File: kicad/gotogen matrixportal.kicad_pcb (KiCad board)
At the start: 2 copper layers, 139.7 x 63.5 mm, 27 parts, among them J1 HUB75 Out, J2 HUB75 In, J3 OLED_128_64, J4 Buttons EXT, J5 OpenMV, J6 Extra Connections, J7 Capacitive Touch, SW1 Back, SW2 Menu, SW3 Up, SW4 Down, SW5 Extra1, SW6 Extra2, U1 MatrixPortal_M4, U2 PCF8523_Breakout, U3 PCF8574, U4 MPR121_Breakout, U5 MAX9814_Breakout

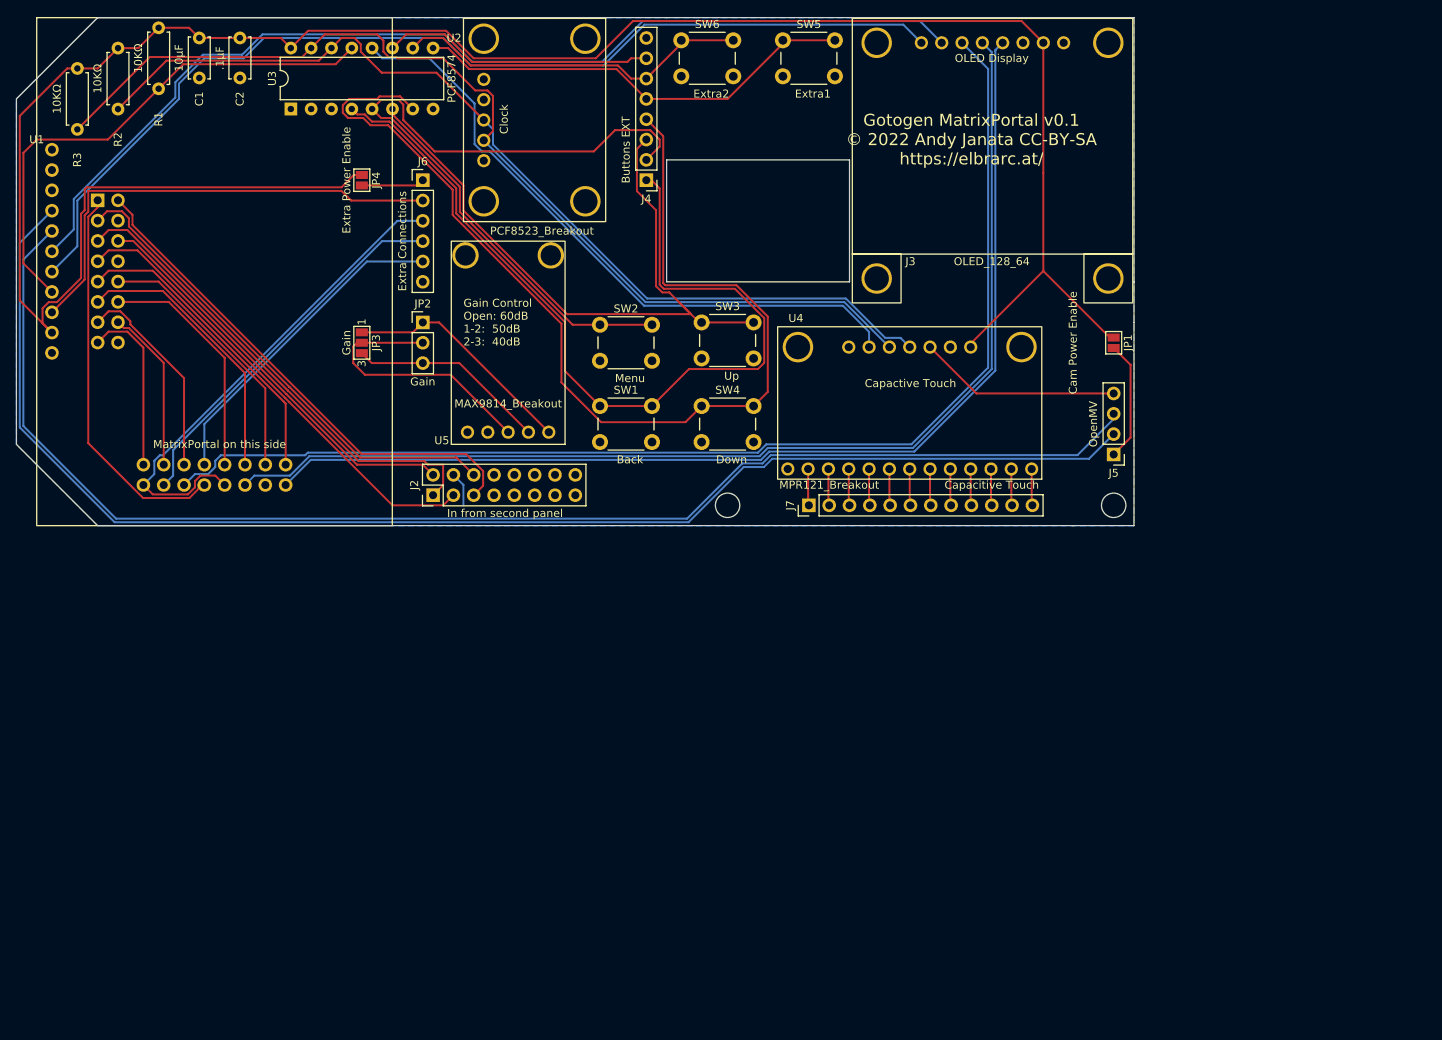
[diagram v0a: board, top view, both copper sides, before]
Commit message: first pass at pcb update
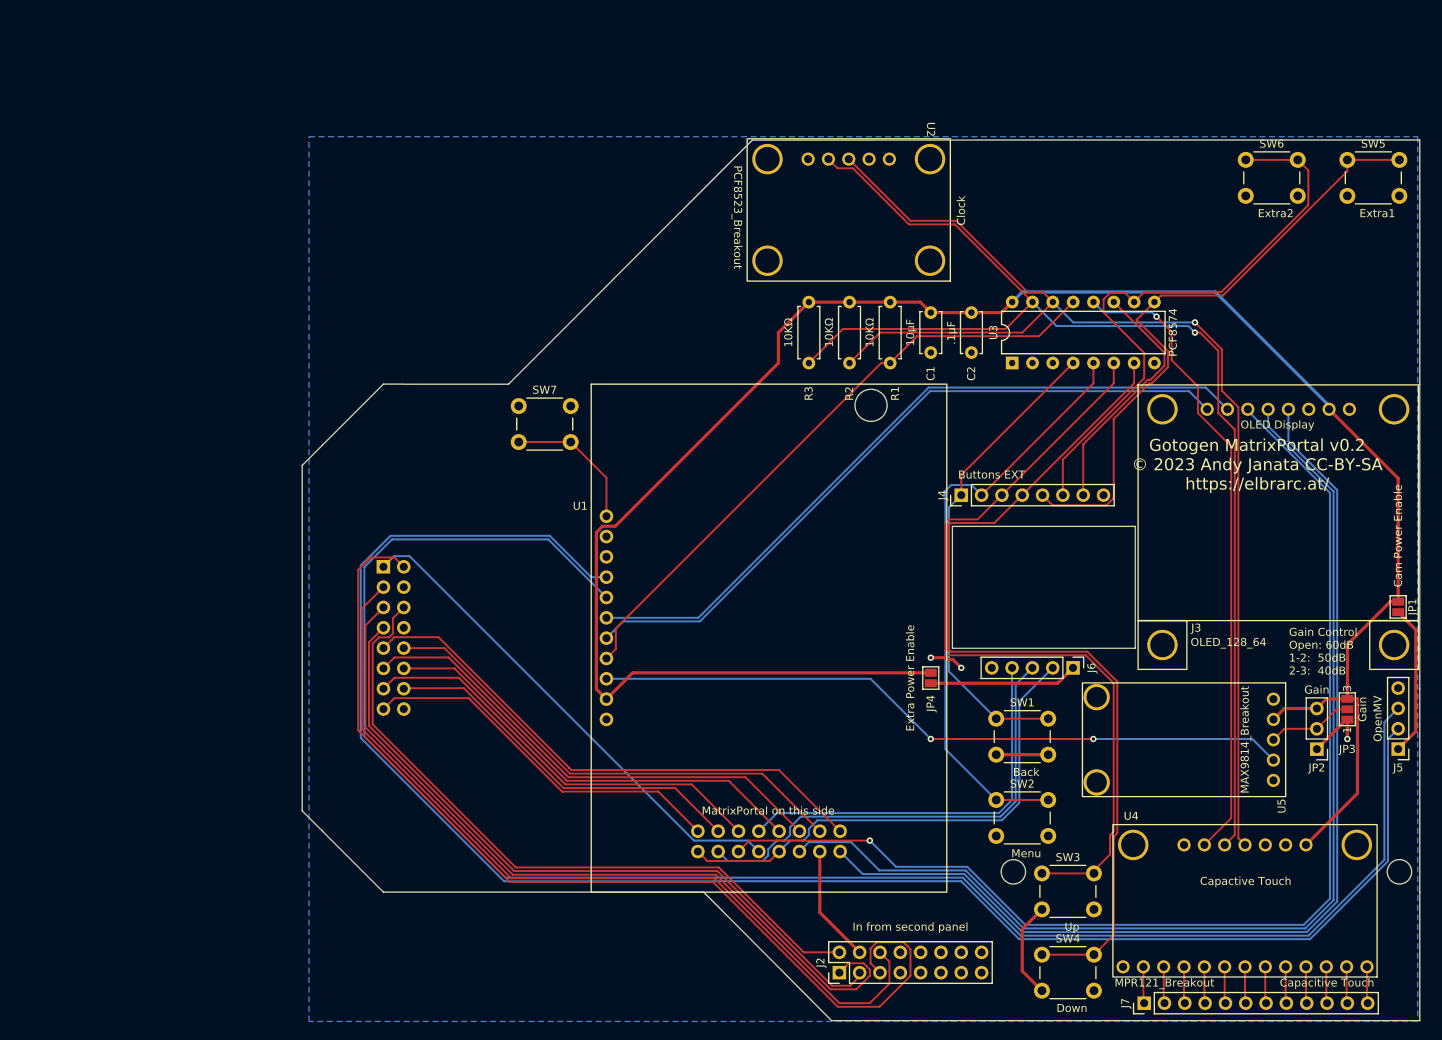
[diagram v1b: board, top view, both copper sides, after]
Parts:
- added SW7: Reset, Button_Switch_THT:SW_PUSH_6mm, F.Cu at (78.0, 66.3)
- J6: footprint Connector_PinHeader_2.54mm:PinHeader_1x06_P2.54mm_Vertical -> Connector_PinHeader_2.54mm:PinHeader_1x05_P2.54mm_Vertical
- moved JP3 131.4 mm to (181.6, 104.2), turned to 90 degrees
- moved JP2 123.8 mm to (177.8, 109.2), turned to 180 degrees
- moved J6 101.6 mm to (147.3, 99.1), turned to -90 degrees
- moved C1 97.7 mm to (129.5, 54.6)
- moved C2 97.7 mm to (134.6, 54.6)
- moved R1 97.7 mm to (124.5, 61.0)
- moved R2 96.8 mm to (119.4, 61.0)
- moved R3 96.0 mm to (114.3, 61.0)
- moved U3 95.6 mm to (139.7, 61.0)
- moved U5 94.9 mm to (173.9, 100.9), turned to -90 degrees
- moved JP4 94.5 mm to (129.5, 100.3)
- moved U1 83.1 mm to (87.1, 63.6)
- moved SW3 81.0 mm to (143.4, 124.8)
- moved SW4 80.7 mm to (143.4, 134.9)
- moved J2 78.4 mm to (118.1, 137.2)
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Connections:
- net /A_GAIN renamed /GAIN
- J6 pad 2: /PA07 -> /PB13
- J6 pad 3: /PB13 -> /PB14
- J6 pad 4: /PB14 -> /PB07
- J6 pad 5: /PB07 -> GND
- JP2 pad 1: /A_GND -> GND
- JP2 pad 3: /A_VDD -> +3.3V
- JP3 pad 1: /A_GND -> GND
- JP3 pad 3: /A_VDD -> +3.3V
- U1 pad 1: unconnected-(U1-Pad1) -> Net-(SW7-Pad2)
- U1 pad 9: /PA07 -> /MIC
- U2 pad 2: unconnected-(U2-Pad2) -> GND
- U5 pad 1: /A_GND -> GND
- U5 pad 2: /A_VDD -> +3.3V
- U5 pad 4: unconnected-(U5-Pad4) -> /MIC
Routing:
- net /MIC: track 0.00 -> 87.6 mm, vias 0 -> 2
- net /LOOP_R2: track 63.9 -> 124.3 mm
- net /PA07: track 59.4 -> 0.00 mm
- net /B_BACK: track 109.1 -> 59.8 mm
- net /CAM_RX: track 172.7 -> 217.2 mm
- net /LOOP_G2: track 61.7 -> 104.4 mm
- net /CAM_TX: track 175.0 -> 215.9 mm
- net /OLED_DATA: track 129.7 -> 88.8 mm
- net /OLED_CLK: track 130.5 -> 90.7 mm
- net /LOOP_R1: track 60.2 -> 98.6 mm
- net /LOOP_G1: track 51.5 -> 87.1 mm
- net /B_EXTRA2: track 44.9 -> 74.9 mm
- net /LOOP_B1: track 58.8 -> 88.7 mm
- net /A_GND: track 29.6 -> 0.00 mm
- net /M_A: track 38.6 -> 67.7 mm
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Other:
- board size 139.7 x 63.5 mm -> 139.7 x 110.1 mm
- board text added: "3V3 PB13 (Out, 5V) PB14 (Out, 5V) PB07 (Out, 5V) GND"
- board text added: "GND Extra 3 Extra 2 Extra 1 Down Up Menu Back"
- board text added: "Gotogen MatrixPortal v0.2 © 2023 Andy Janata CC-BY-SA https://elbrarc.at/"
- board text removed: "3V3 PA07 (I/O, 3V3) PB13 (Out, 5V) PB14 (Out, 5V) PB07 (Out, 5V) GND"
- board text removed: "GND -- Extra 3 Extra 2 Extra 1 Down Up Menu Back"
- board text removed: "Gotogen MatrixPortal v0.1 © 2022 Andy Janata CC-BY-SA https://elbrarc.at/"

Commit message: further pcb updates
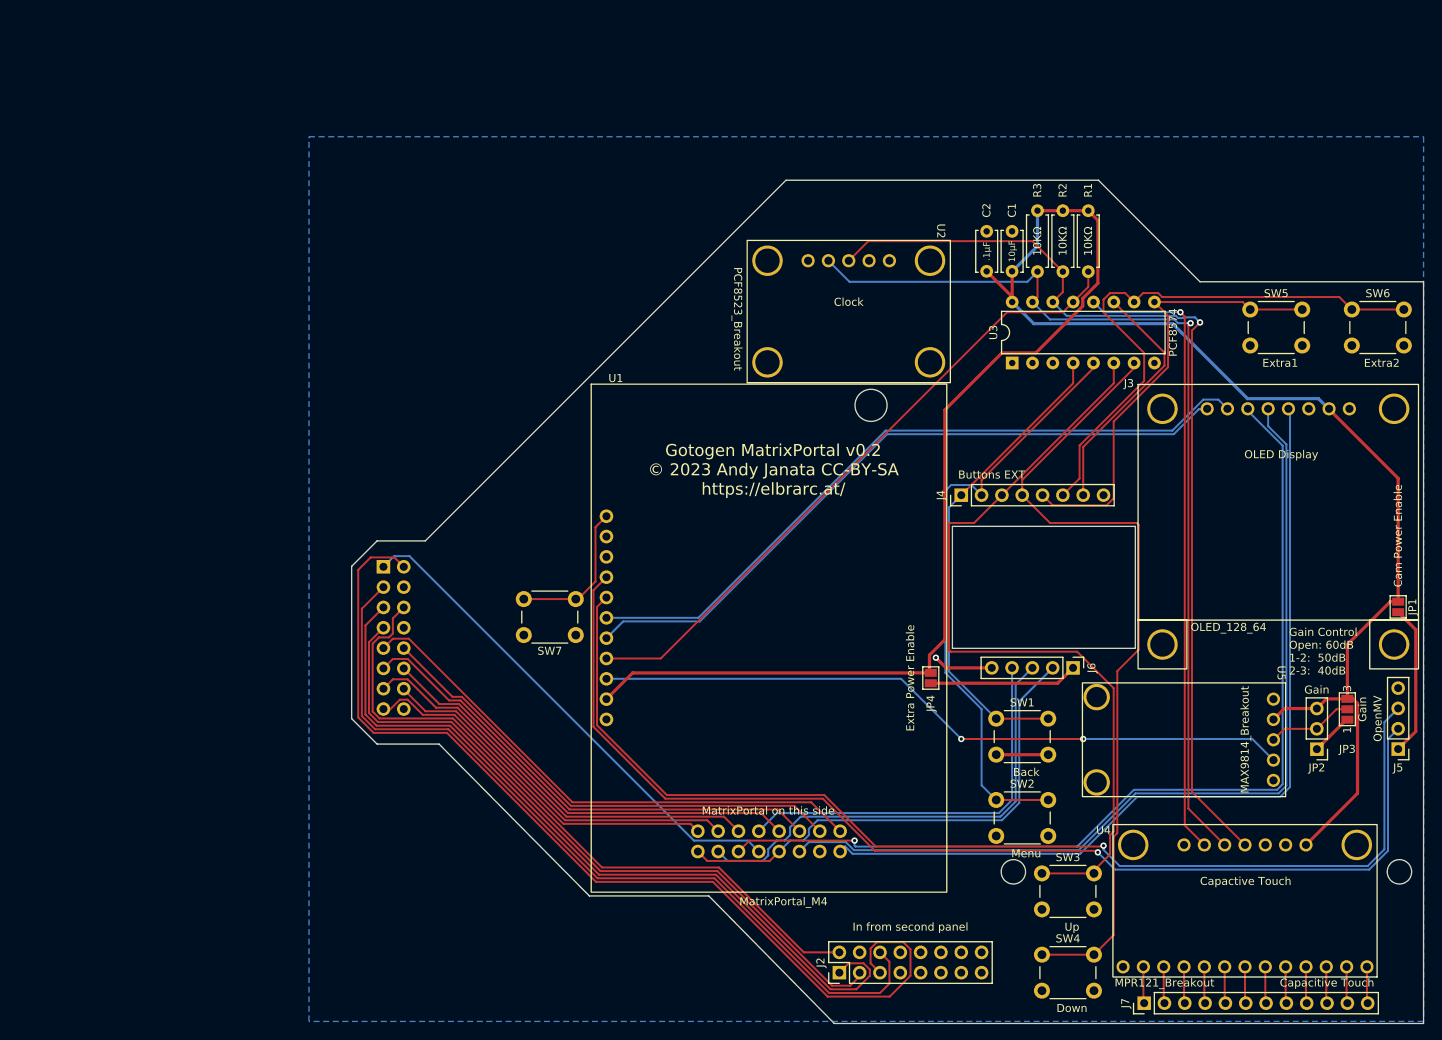
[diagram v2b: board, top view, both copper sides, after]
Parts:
- moved R3 30.8 mm to (142.9, 49.5)
- moved SW7 29.5 mm to (85.2, 95.0), turned to 180 degrees
- moved R2 29.0 mm to (146.1, 49.5)
- moved R1 27.3 mm to (149.2, 49.5)
- moved SW6 22.9 mm to (182.2, 54.3)
- moved SW5 22.3 mm to (169.5, 54.3)
- moved U2 12.7 mm to (132.0, 63.4)
- moved C1 11.4 mm to (139.7, 49.5), turned to 90 degrees
- moved C2 5.50 mm to (136.5, 49.5), turned to 90 degrees
- moved J3 0.06 mm to (155.5, 63.6)
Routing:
- net /CAM_RX: track 217.2 -> 141.7 mm, vias 0 -> 1
- net /CAM_TX: track 215.9 -> 142.8 mm, vias 0 -> 1
- net /I2C_SDA: track 152.9 -> 119.9 mm
- net /I2C_SCL: track 148.2 -> 121.7 mm
- net GND: track 45.5 -> 19.3 mm, vias 3 -> 1
- net /OLED_RST: track 137.9 -> 113.1 mm
- net /OLED_DC: track 145.6 -> 121.2 mm
- net /OLED_CS: track 131.9 -> 107.6 mm
- net /B_EXTRA1: track 78.7 -> 56.7 mm
- net /B_DOWN: track 113.1 -> 100.9 mm
- net /B_EXTRA2: track 74.9 -> 70.4 mm
- net +3.3V: track 252.4 -> 256.0 mm
- net /GPIO_INT: track 78.3 -> 81.4 mm
- net /LOOP_G2: track 104.4 -> 102.4 mm
- net /LOOP_R2: track 124.3 -> 122.3 mm
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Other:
- board size 139.7 x 110.1 mm -> 134 x 105.4 mm
